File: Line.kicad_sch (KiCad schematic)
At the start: 50 parts, among them U0 QRE1113GR, U1 QRE1113GR, U10 QRE1113GR, U11 QRE1113GR, U12 QRE1113GR, U13 QRE1113GR, U14 QRE1113GR, U16 CD74HC4067M, U2 QRE1113GR, U3 QRE1113GR, U4 QRE1113GR, U5 QRE1113GR, U6 QRE1113GR, U7 QRE1113GR, U8 QRE1113GR, U9 QRE1113GR

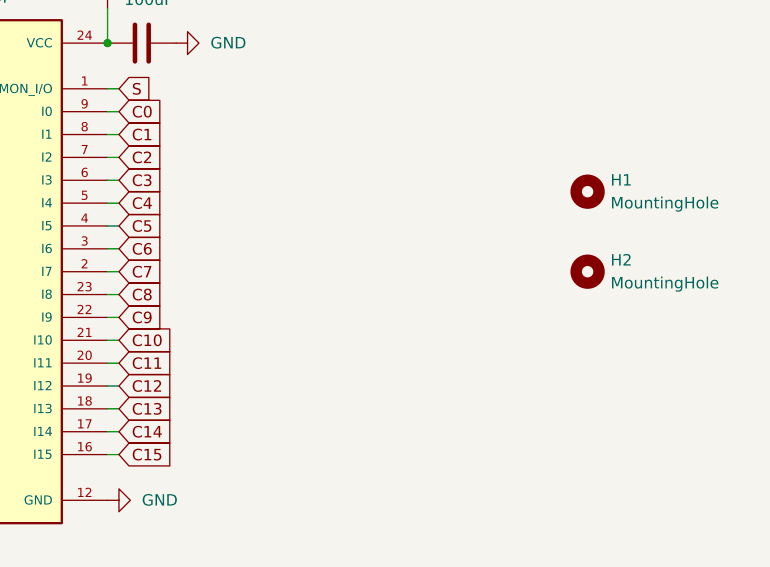
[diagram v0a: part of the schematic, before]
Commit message: đon
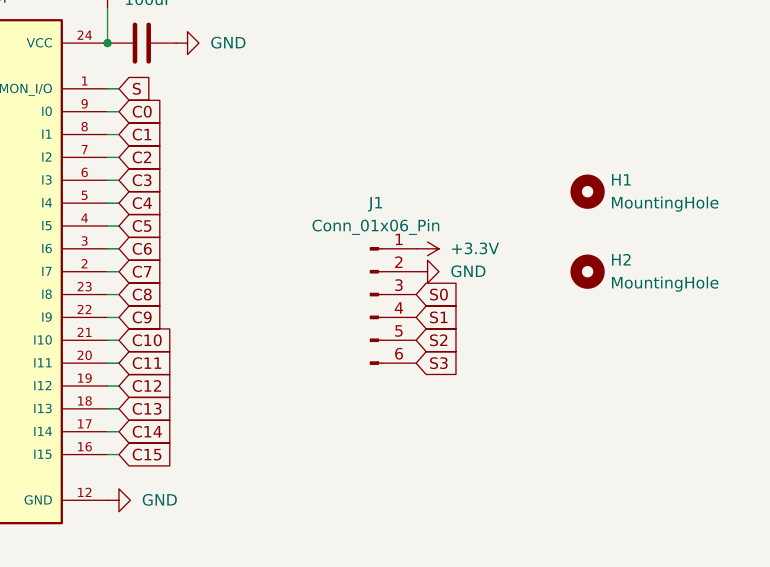
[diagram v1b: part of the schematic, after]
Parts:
- added J1: Conn_01x06_Pin, Connector_JST:JST_ZH_B6B-ZR_1x06_P1.50mm_Vertical, symbol Connector:Conn_01x06_Pin
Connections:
- net +3.3V: now also J1.1 (Pin_1)
- net GND: now also J1.2 (Pin_2)
- net S0: now also J1.3 (Pin_3)
- net S1: now also J1.4 (Pin_4)
- net S2: now also J1.5 (Pin_5)
- net S3: now also J1.6 (Pin_6)
